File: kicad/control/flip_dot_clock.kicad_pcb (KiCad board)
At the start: 4 copper layers, 140.2 x 46.1 mm, 34 parts, among them J1 Conn_01x02_Male, U1 NUCLEO-F303K8-HEADER, U10 Small_7_Seg_FlipDot_Module, U2 SLC03B-05, U3 NCV7719, U4 Small_7_Seg_FlipDot_Module, U5 NCV7719, U6 Small_7_Seg_FlipDot_Module, U7 NCV7719, U8 Small_7_Seg_FlipDot_Module, U9 NCV7719

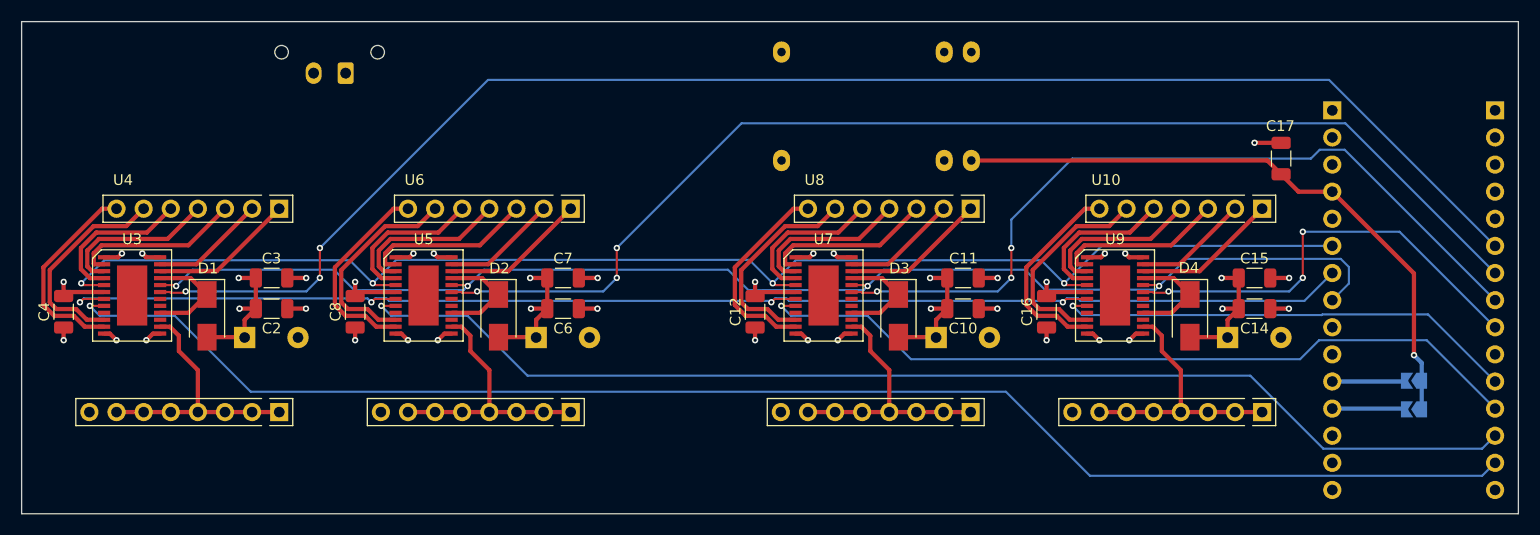
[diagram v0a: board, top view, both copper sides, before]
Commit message: update pcb
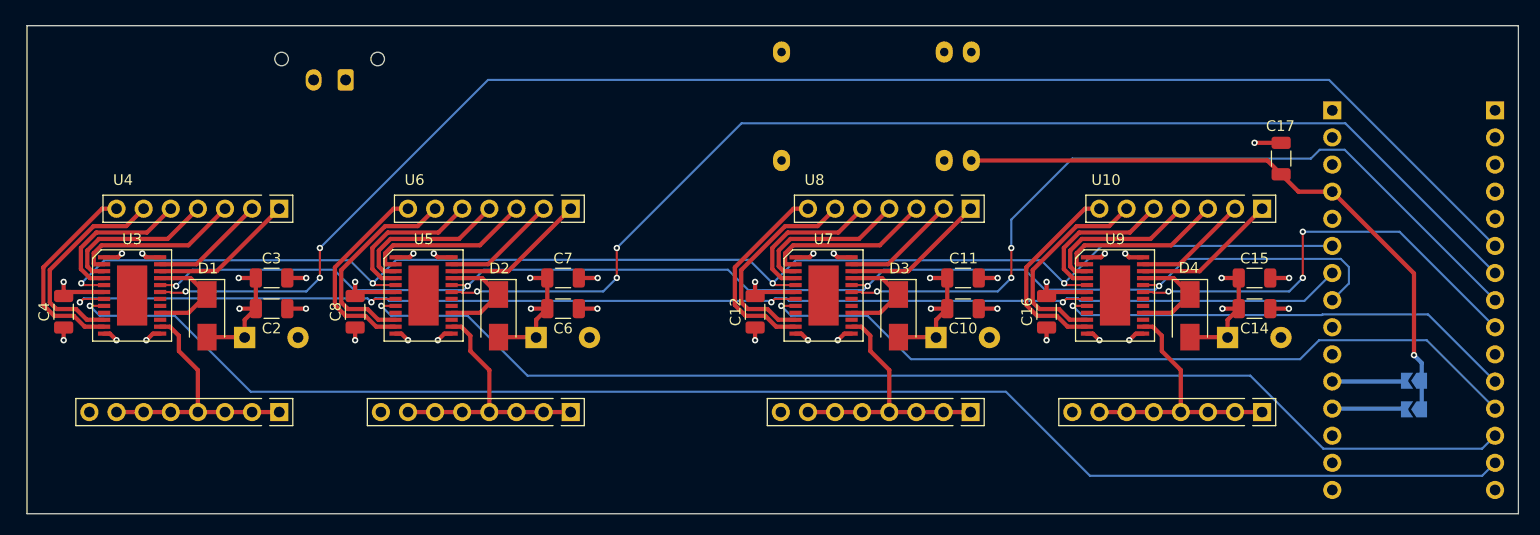
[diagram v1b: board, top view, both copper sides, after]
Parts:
- moved J1 0.63 mm to (109.1, 78.7)
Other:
- board size 140.2 x 46.1 mm -> 139.7 x 45.7 mm
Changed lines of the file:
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@@
     )
     (pad_to_mask_clearance 0)
-    (grid_origin 78.74 119.38)
+    (grid_origin 79.248 119.38)
     (pcbplotparams
       (layerselection 0x00010f0_ffffffff)
@@
       (effects (font (size 1 1) (thickness 0.15)))
     )
-    (fp_text value "Small_7_Seg_FlipDot_Module" (at 12.7 -15.875) (layer "F.Fab")
+    (fp_text value "Small_7_Seg_FlipDot_Module" (at 12.573 -4.064) (layer "F.Fab")
       (effects (font (size 1 1) (thickness 0.15)))
     )
@@
       (effects (font (size 1 1) (thickness 0.15)))
     )
-    (fp_text value "Small_7_Seg_FlipDot_Module" (at 12.7 -15.875) (layer "F.Fab")
+    (fp_text value "Small_7_Seg_FlipDot_Module" (at 12.573 -4.064) (layer "F.Fab")
       (effects (font (size 1 1) (thickness 0.15)))
     )
@@
       (effects (font (size 1 1) (thickness 0.15)))
     )
-    (fp_text value "Small_7_Seg_FlipDot_Module" (at 12.7 -15.875) (layer "F.Fab")
+    (fp_text value "Small_7_Seg_FlipDot_Module" (at 12.573 -4.064) (layer "F.Fab")
       (effects (font (size 1 1) (thickness 0.15)))
     )
@@
       (effects (font (size 1 1) (thickness 0.15)))
     )
-    (fp_text value "Small_7_Seg_FlipDot_Module" (at 12.7 -15.875) (layer "F.Fab")
+    (fp_text value "Small_7_Seg_FlipDot_Module" (at 12.7 -4.191) (layer "F.Fab")
       (effects (font (size 1 1) (thickness 0.15)))
     )
@@
   )
   (footprint "Connector_Molex:Molex_Micro-Fit_3.0_43650-0215_1x02_P3.00mm_Vertical" (layer "B.Cu")
-    (at 109.093 78.105 180)
+    (at 109.093 78.74 180)
     (descr "Molex Micro-Fit 3.0 Connector System, 43650-0215 (compatible alternatives: 43650-0216, 43650-0217), 2 Pins per row (http://www.molex.com/pdm_docs/sd/436500215_sd.pdf), generated with kicad-footprint-generator")
     (tags "connector Molex Micro-Fit_3.0 vertical")
@@
     )
   )
-  (gr_line (start 78.74 119.38) (end 78.74 73.279)
+  (gr_line (start 79.248 119.38) (end 79.248 73.66)
     (stroke (width 0.05) (type solid)) (layer "Edge.Cuts"))
-  (gr_line (start 78.74 73.279) (end 218.948 73.279)
+  (gr_line (start 79.248 73.66) (end 218.948 73.66)
     (stroke (width 0.05) (type solid)) (layer "Edge.Cuts"))
-  (gr_line (start 218.948 119.38) (end 78.74 119.38)
+  (gr_line (start 218.948 119.38) (end 79.248 119.38)
     (stroke (width 0.05) (type solid)) (layer "Edge.Cuts"))
-  (gr_line (start 218.948 73.279) (end 218.948 119.38)
+  (gr_line (start 218.948 73.66) (end 218.948 119.38)
     (stroke (width 0.05) (type solid)) (layer "Edge.Cuts"))
+  (dimension (type aligned) (layer "Eco1.User")
+    (pts (xy 79.248 119.38) (xy 218.948 119.38))
+    (height 8.762999)
+    (gr_text "5500.0000  mils" (at 149.098 126.342999) (layer "Eco1.User")
+      (effects (font (size 1.5 1.5) (thickness 0.3)))
+    )
+    (format (units 3) (units_format 1) (precision 4))
+    (style (thickness 0.2) (arrow_length 1.27) (text_position_mode 0) (extension_height 0.58642) (extension_offset 0.5) keep_text_aligned)
+  )
+  (dimension (type aligned) (layer "Eco1.User")
+    (pts (xy 79.248 119.38) (xy 79.248 73.66))
+    (height -6.858)
+    (gr_text "1800.0000  mils" (at 70.59 96.52 90) (layer "Eco1.User")
+      (effects (font (size 1.5 1.5) (thickness 0.3)))
+    )
+    (format (units 3) (units_format 1) (precision 4))
+    (style (thickness 0.2) (arrow_length 1.27) (text_position_mode 0) (extension_height 0.58642) (extension_offset 0.5) keep_text_aligned)
+  )
   (segment (start 96.107 98.838) (end 94.577 97.308) (width 0.4) (layer "F.Cu") (net 1))
   (segment (start 96.107 98.838) (end 94.387 100.558) (width 0.4) (layer "F.Cu") (net 1))
@@
       (pts
         (xy 218.44 118.872)
-        (xy 79.248 118.872)
-        (xy 79.248 73.787)
-        (xy 218.44 73.787)
+        (xy 79.756 118.872)
+        (xy 79.756 74.168)
+        (xy 218.44 74.168)
       )
     )
@@
         (xy 86.106 94.996)
         (xy 86.106 99.441)
-        (xy 79.248 99.441)
-        (xy 79.248 90.043)
+        (xy 79.756 99.441)
+        (xy 79.756 90.043)
         (xy 86.106 90.043)
         (xy 86.106 92.329)
@@
       (pts
         (xy 218.44 118.872)
-        (xy 79.248 118.872)
-        (xy 79.248 100.076)
+        (xy 79.756 118.872)
+        (xy 79.756 100.076)
         (xy 86.741 100.076)
         (xy 86.741 95.631)
@@
         (xy 162.179 82.55)
         (xy 162.179 89.281)
-        (xy 79.248 89.408)
-        (xy 79.248 73.787)
-        (xy 166.751 73.787)
-        (xy 218.44 73.787)
+        (xy 79.756 89.408)
+        (xy 79.756 74.168)
+        (xy 218.44 74.168)
       )
     )
